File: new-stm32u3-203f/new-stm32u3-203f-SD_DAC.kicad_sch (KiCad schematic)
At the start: 11 parts, among them J1 DM3CS-SF, J2 SJ-3524-SMT, U2 TLV320DAC3203IRGER

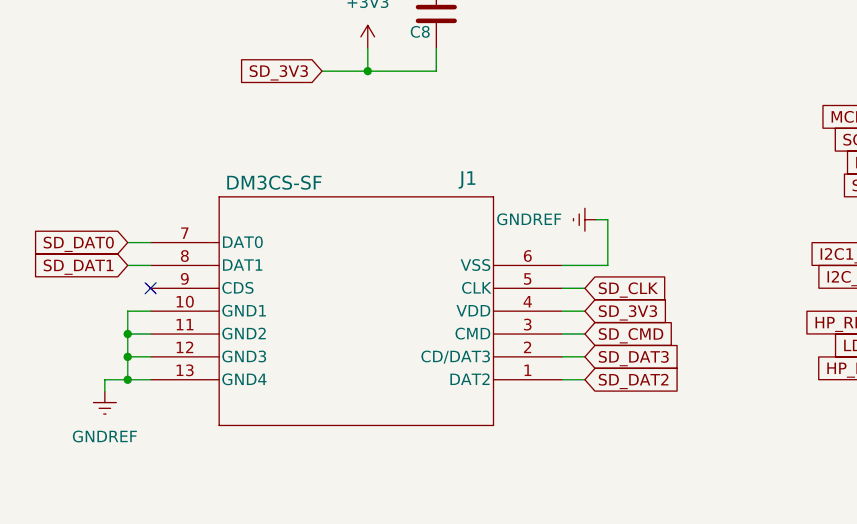
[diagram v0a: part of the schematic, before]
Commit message: moved over to new sd card stuff
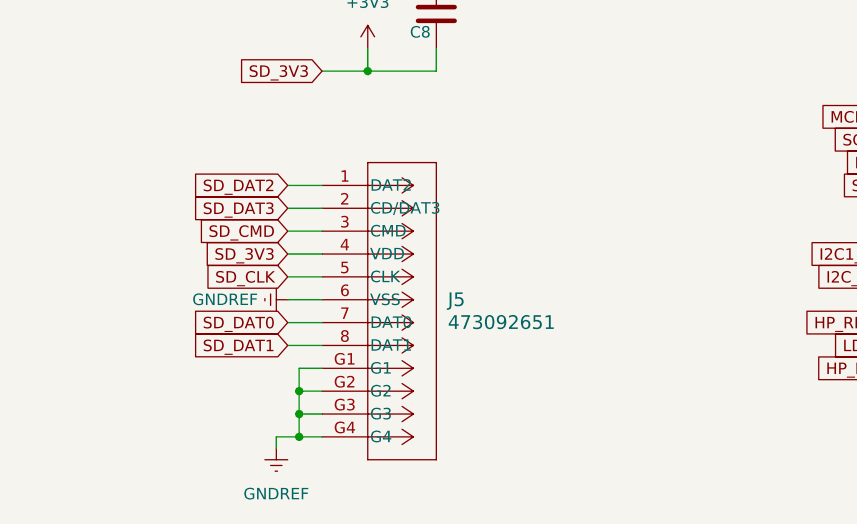
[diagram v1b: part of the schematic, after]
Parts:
- removed J1: DM3CS-SF, DM3CS-SF_HIR, symbol 2026-01-24_09-53-21:DM3CS-SF
- added J5: 473092651, CONN12_47309-2651_MOL, symbol 2026-01-28_06-17-02:473092651
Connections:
- net +3V3: now also J5.4 (VDD)
- net GNDREF: now also J5.6 (VSS), J5.G1, J5.G2, J5.G3, J5.G4
- net SD_CLK: now also J5.5 (CLK)
- net SD_CMD: now also J5.3 (CMD)
- net SD_DAT0: now also J5.7 (DAT0)
- net SD_DAT1: now also J5.8 (DAT1)
- net SD_DAT2: now also J5.1 (DAT2)
- net SD_DAT3: now also J5.2 (CD/DAT3)
- no-connect marks 4 -> 3
